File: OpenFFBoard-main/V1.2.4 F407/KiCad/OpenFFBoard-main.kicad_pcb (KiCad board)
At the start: 2 copper layers, 60 x 60 mm, 66 parts, among them J1 USB4105-GF-A, SW1 TL3342F160QG/TR, SW2 TL3342F160QG/TR, U1 STM32F407VGT6, U2 TJA1051T/3, U3 LM1117, U4 USBLC6-2SC6, X1 8MHz

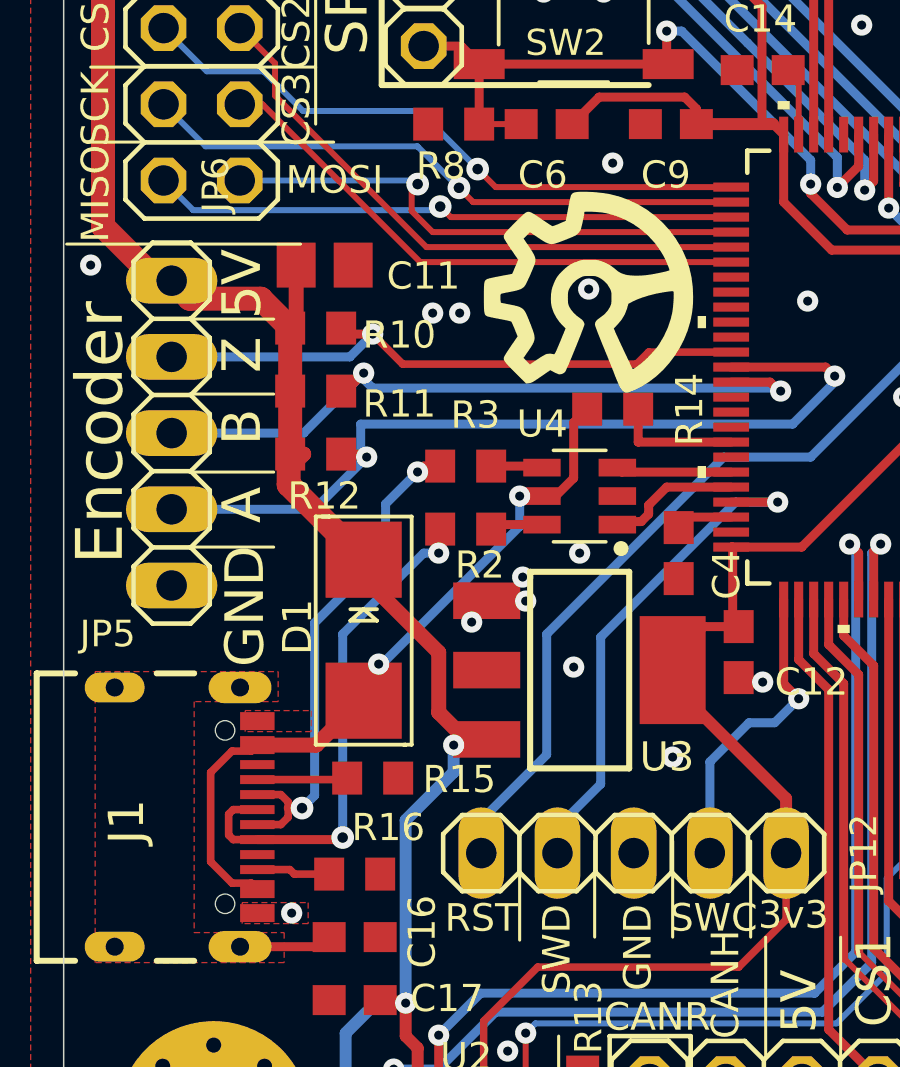
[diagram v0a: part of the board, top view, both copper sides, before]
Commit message: Generated manufacturing files
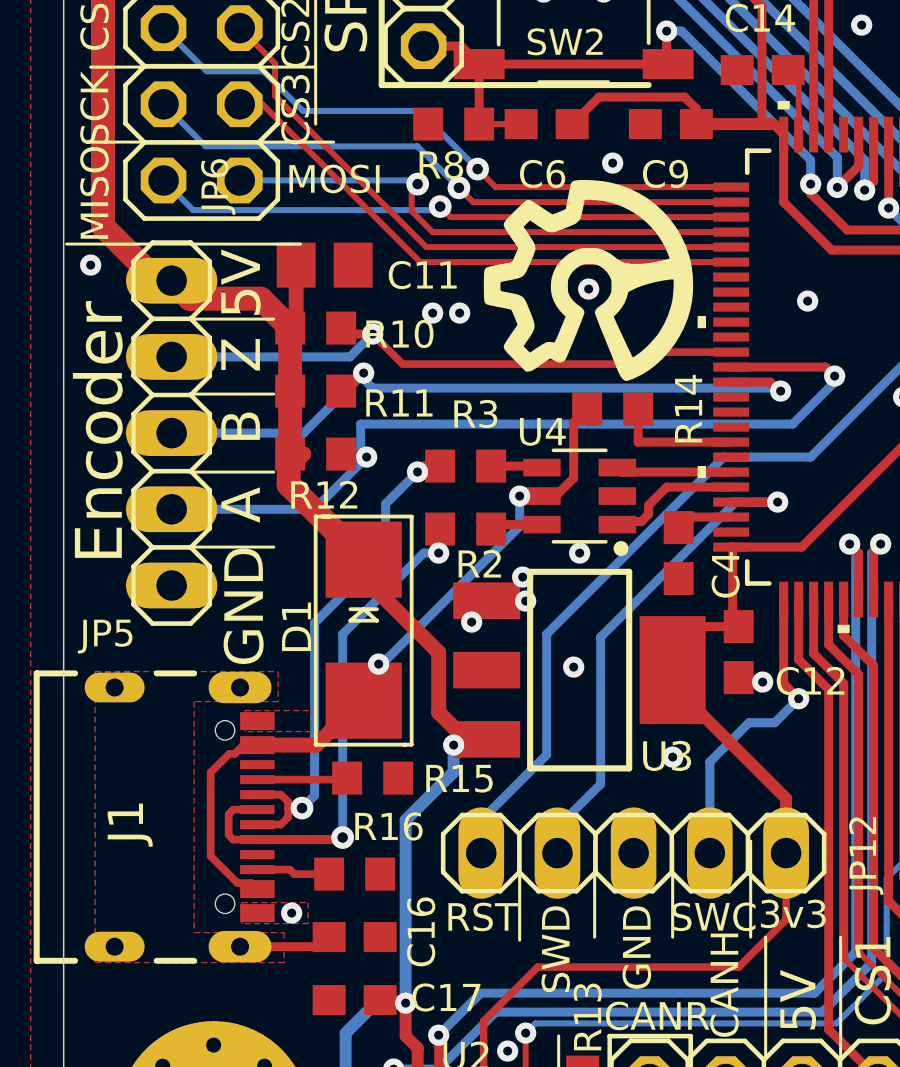
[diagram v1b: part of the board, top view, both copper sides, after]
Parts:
- moved G*** 0.39 mm to (136.0, 102.1)
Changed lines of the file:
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@@
       (layerselection 0x00010fc_ffffffff)
       (disableapertmacros false)
-      (usegerberextensions false)
-      (usegerberattributes true)
-      (usegerberadvancedattributes true)
-      (creategerberjobfile true)
+      (usegerberextensions true)
+      (usegerberattributes false)
+      (usegerberadvancedattributes false)
+      (creategerberjobfile false)
       (svguseinch false)
       (svgprecision 6)
@@
       (psa4output false)
       (plotreference true)
-      (plotvalue true)
+      (plotvalue false)
       (plotinvisibletext false)
       (sketchpadsonfab false)
-      (subtractmaskfromsilk false)
+      (subtractmaskfromsilk true)
       (outputformat 1)
       (mirror false)
-      (drillshape 1)
+      (drillshape 0)
       (scaleselection 1)
-      (outputdirectory "")
+      (outputdirectory "Manufacturing/")
     )
   )
@@
   )
   (footprint "LOGO" (layer "F.Cu")
-    (at 136 102.5)
+    (at 136 102.108)
     (attr board_only exclude_from_pos_files exclude_from_bom)
     (fp_text reference "G***" (at 0 0) (layer "F.SilkS") hide
@@
     (property "Sheetfile" "File: OpenFFBoard-main.kicad_sch")
     (property "Sheetname" "")
-    (fp_text reference "U4" (at 2.1011 2.4036) (layer "F.SilkS")
+    (fp_text reference "U4" (at 2.0971 2.1156) (layer "F.SilkS")
       (effects (font (size 0.906528 0.906528) (thickness 0.093472)) (justify left))
     )
@@
   (segment (start 127.3511 124.0036) (end 127.0311 124.3236) (width 0.3) (layer "F.Cu") (net 9))
   (segment (start 127.0311 124.3236) (end 124.3811 124.3236) (width 0.3) (layer "F.Cu") (net 9))
+  (segment (start 124.7561 122.2036) (end 124.297017 122.2036) (width 0.254) (layer "F.Cu") (net 10))
+  (segment (start 124.021167 117.895601) (end 124.205016 117.895601) (width 0.254) (layer "F.Cu") (net 10))
   (segment (start 129.0011 114.9036) (end 129.0011 115.6231) (width 0.3) (layer "F.Cu") (net 10))
   (segment (start 124.9561 122.4036) (end 124.7561 122.2036) (width 0.254) (layer "F.Cu") (net 10))
+  (segment (start 124.205016 117.895601) (end 124.497017 117.6036) (width 0.254) (layer "F.Cu") (net 10))
   (segment (start 134.9011 109.3036) (end 133.7011 109.3036) (width 0.3) (layer "F.Cu") (net 10))
   (segment (start 128.4011 116.1231) (end 128.5011 116.1231) (width 0.5) (layer "F.Cu") (net 10))
-  (segment (start 124.7561 117.8036) (end 124.113168 117.8036) (width 0.254) (layer "F.Cu") (net 10))
+  (segment (start 123.4011 118.515668) (end 124.021167 117.895601) (width 0.254) (layer "F.Cu") (net 10))
   (segment (start 135.5011 106.8536) (end 135.5011 108.7036) (width 0.3) (layer "F.Cu") (net 10))
-  (segment (start 124.7561 117.8036) (end 124.9561 117.6036) (width 0.254) (layer "F.Cu") (net 10))
   (segment (start 135.5011 106.8536) (end 135.9511 106.4036) (width 0.3) (layer "F.Cu") (net 10))
-  (segment (start 123.4011 118.515668) (end 124.113168 117.8036) (width 0.254) (layer "F.Cu") (net 10))
   (segment (start 124.9561 117.6036) (end 126.9206 117.6036) (width 0.5) (layer "F.Cu") (net 10))
-  (segment (start 124.7561 122.2036) (end 124.113168 122.2036) (width 0.254) (layer "F.Cu") (net 10))
+  (segment (start 124.497017 117.6036) (end 124.9561 117.6036) (width 0.254) (layer "F.Cu") (net 10))
   (segment (start 135.5011 108.7036) (end 134.9011 109.3036) (width 0.3) (layer "F.Cu") (net 10))
   (segment (start 128.4011 116.1231) (end 126.9206 117.6036) (width 0.5) (layer "F.Cu") (net 10))
-  (segment (start 124.113168 122.2036) (end 123.4011 121.491531) (width 0.254) (layer "F.Cu") (net 10))
   (segment (start 134.4448 109.3036) (end 133.7011 109.3036) (width 0.4) (layer "F.Cu") (net 10))
-  (segment (start 123.4011 121.491531) (end 123.4011 118.515668) (width 0.254) (layer "F.Cu") (net 10))
+  (segment (start 124.297017 122.2036) (end 123.4011 121.307683) (width 0.254) (layer "F.Cu") (net 10))
+  (segment (start 123.4011 121.307683) (end 123.4011 118.515668) (width 0.254) (layer "F.Cu") (net 10))
   (segment (start 128.5011 116.1231) (end 129.0011 115.6231) (width 0.3) (layer "F.Cu") (net 10))
   (via (at 133.7011 109.3036) (size 0.7064) (drill 0.3) (layers "F.Cu" "B.Cu") (net 10))
